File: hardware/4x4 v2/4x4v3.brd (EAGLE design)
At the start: 89.2 x 36.7 mm, 59 parts, among them IC1 PIC18F2480-I/SP, J1 USB1035-XX-X-X-X-B_REVE, T1 BC547, T2 BC547, T3 BC547, T4 BC547, U1 IR3315, U2 IR3315, U3 IR3315, U4 IR3315

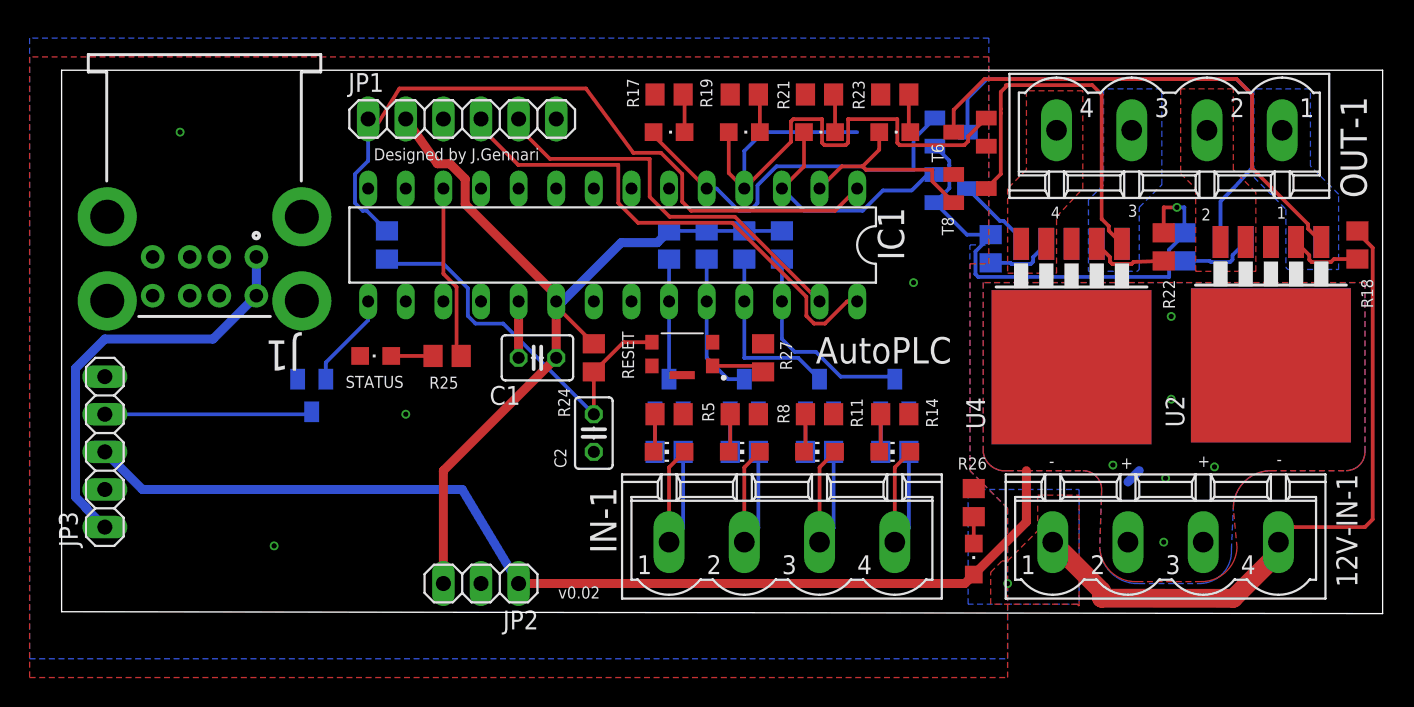
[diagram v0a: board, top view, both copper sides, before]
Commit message: Rev
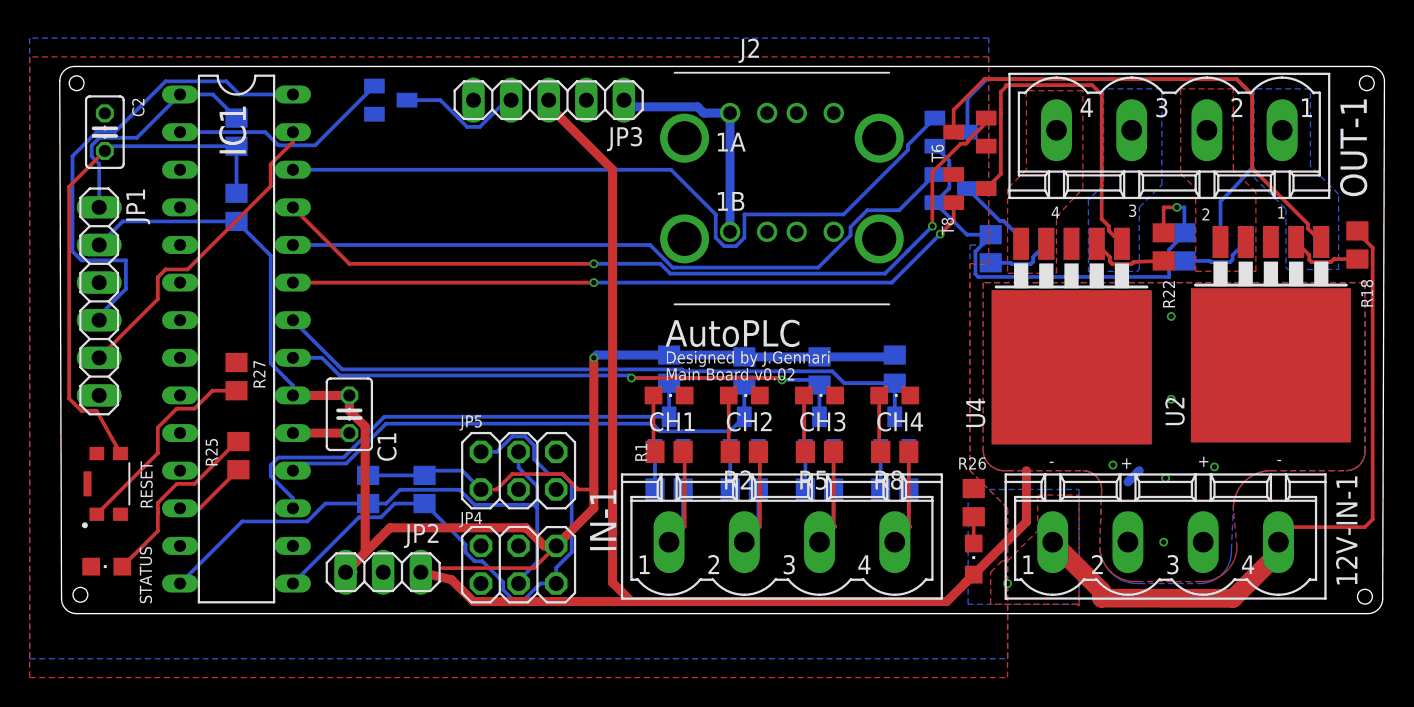
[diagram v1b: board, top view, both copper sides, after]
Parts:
- removed J1: USB1035-XX-X-X-X-B_REVE, USB1035-XX-X-X-X-B_REVE:GCT_USB1035-XX-X-X-X-B_REVE
- removed LED4: (no value), led:CHIP-LED0805
- removed LED6, LED7, LED8: (no value), led:CHIPLED_0805
- removed R11: 680, resistor:R0805
- removed R19, R21, R23: 150R, resistor:R0805
- added J2: (no value), InputOutputIO (rev17e):614008235023
- added JP4, JP5: (no value), pinhead:2X03
- added R1, R2: (no value), resistor:R0805
- LED1: value 12123 -> (none); device led:CHIP-LED0805 -> led:CHIPLED_0805
- LED2, LED3: device led:CHIP-LED0805 -> led:CHIPLED_0805
- R14, R5, R8: value 680 -> (none)
- R17: value 150R -> (none)
- moved S1 39.7 mm to (26.9, 22.0), turned to 90 degrees
- moved C2 38.8 mm to (26.7, 45.7), turned to 90 degrees
- moved JP3 38.2 mm to (56.6, 47.9), turned to 180 degrees
- moved R27 35.6 mm to (35.6, 29.2)
- moved R17 33.5 mm to (44.5, 21.6), flipped to the bottom, turned to 90 degrees
- moved R14 32.2 mm to (48.3, 21.6), flipped to the bottom, turned to 270 degrees
- moved JP1 27.4 mm to (26.3, 34.3), turned to 270 degrees
- moved IC1 26.2 mm to (35.6, 31.8), turned to 270 degrees
- moved R24 26.2 mm to (35.6, 40.6), flipped to the bottom, turned to 270 degrees
- moved LED9 23.1 mm to (26.8, 16.4)
- moved T9 20.6 mm to (46.0, 47.9), turned to 90 degrees
- moved LED5 17.8 mm to (64.8, 27.9)
- moved R25 15.6 mm to (35.7, 23.9), turned to 90 degrees
- moved C1 13.3 mm to (43.2, 26.7), turned to 270 degrees
- moved R3 12.7 mm to (35.6, 45.7)
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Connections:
- removed net N$11: LED4.C, R14.1
- removed net N$14: LED5.C, R17.2
- removed net N$17: LED6.C, R19.2
- removed net N$20: LED7.C, R21.2
- removed net N$23: LED8.C, R23.2
- new net N$3: LED5.A, R1.2
- new net SCL: IC1.14, JP4.4, JP5.4, R17.1
- new net SDA: IC1.15, JP4.2, JP5.2, R14.2
- net GND: now also J2.A4, J2.B4, J2.SHELL, J2.SHELL1, J2.SHELL2, J2.SHELL3, JP4.3, JP5.3, LED1.C, LED2.C, LED3.C, LED5.C; no longer J1.10, J1.11, J1.12, J1.4A, J1.4B, J1.9, R11.2, R14.2, R17.1, R19.1, R21.1, R23.1, R5.2, R8.2
- net IN-1-1: now also R1.1; no longer LED1.A
- net IN-1-2: now also R2.1; no longer LED2.A
- net IN-1-3: now also R5.1; no longer LED3.A
- net IN-1-4: now also R8.1; no longer LED4.A
- net N$5: now also LED1.A, R2.2; no longer LED1.C, R5.1
- net N$7: now also LED2.A, R5.2; no longer LED2.C, R8.1
- net N$9: now also LED3.A, R8.2; no longer LED3.C, R11.1
- net OUT-1-5: now also J2.A1, J2.B1; no longer J1.1A, J1.1B
- net SIGIN-1-1: now also IC1.17; no longer IC1.23
- net SIGIN-1-2: now also IC1.18; no longer IC1.24
- net SIGIN-1-3: now also IC1.21; no longer IC1.25
- net SIGIN-1-4: now also IC1.22; no longer IC1.26
- net SIGOUT-1-1: now also IC1.26; no longer IC1.5, LED5.A
- net SIGOUT-1-2: now also IC1.25; no longer IC1.4, LED6.A
- net SIGOUT-1-3: now also IC1.24; no longer IC1.3, LED7.A
- net SIGOUT-1-4: now also IC1.23; no longer IC1.2, LED8.A
- net SIGOUT-1-5: now also IC1.2; no longer IC1.15
- net VCC: now also JP4.1, JP5.1, R14.1, R17.2
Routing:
- net VCC: track 60.1 -> 115.8 mm, vias 0 -> 1
- net SDA: track 0.00 -> 39.3 mm
- net SCL: track 0.00 -> 37.2 mm
- net SIGOUT-1-4: track 13.9 -> 47.6 mm, vias 0 -> 2
- net MCLR: track 49.8 -> 16.3 mm
- net SIGIN-1-4: track 14.1 -> 44.7 mm
- net SIGOUT-1-3: track 16.4 -> 46.9 mm
- net SIGIN-1-3: track 12.3 -> 38.5 mm, vias 0 -> 2
- net SIGIN-1-1: track 8.11 -> 34.1 mm
- net SIGOUT-1-1: track 26.0 -> 51.1 mm
- net SIGIN-1-2: track 9.81 -> 34.6 mm
- net SIGOUT-1-2: track 40.0 -> 55.4 mm, vias 0 -> 2
- net OUT-1-5: track 28.4 -> 15.5 mm
- net 12V-1: track 73.1 -> 85.4 mm
- net N$2: track 3.98 -> 13.9 mm
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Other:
- board size 89.2 x 36.7 mm -> 89.5 x 36.9 mm
- board text added: "CH1"
- board text added: "CH2"
- board text added: "CH3"
- board text added: "CH4"
- board text added: "Main Board v0.02"
- board text removed: "v0.02"
